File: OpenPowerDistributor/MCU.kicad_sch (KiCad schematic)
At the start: 1 part, among them U15 ESP32-S2-WROVER

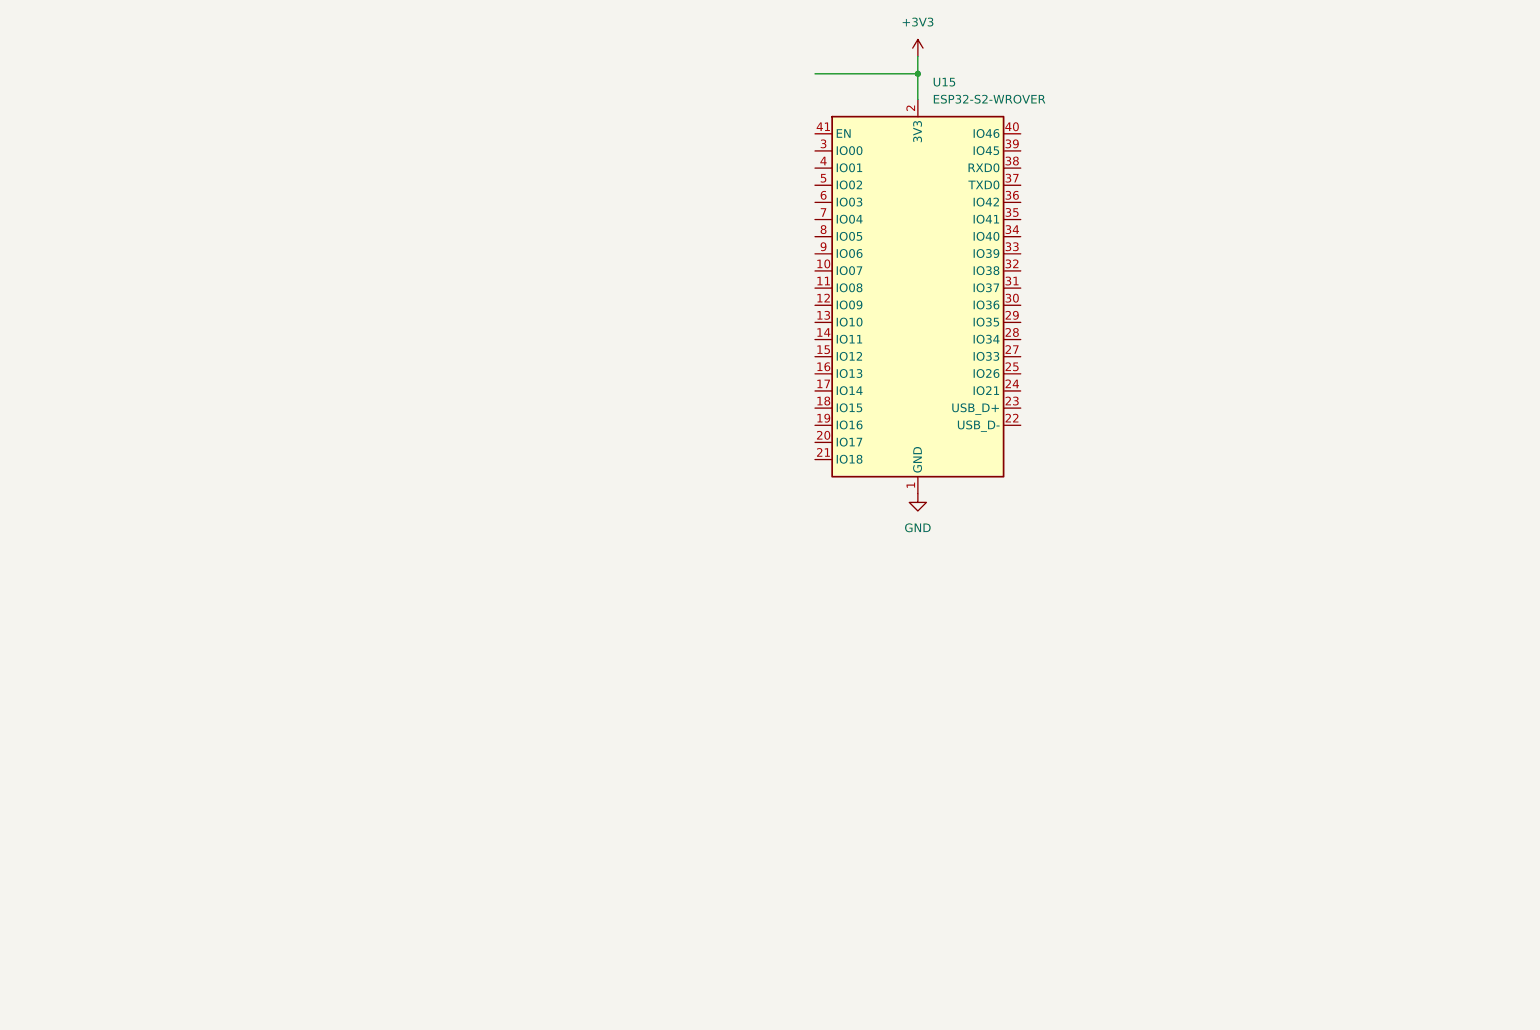
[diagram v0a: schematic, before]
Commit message: Analog multiplexer work
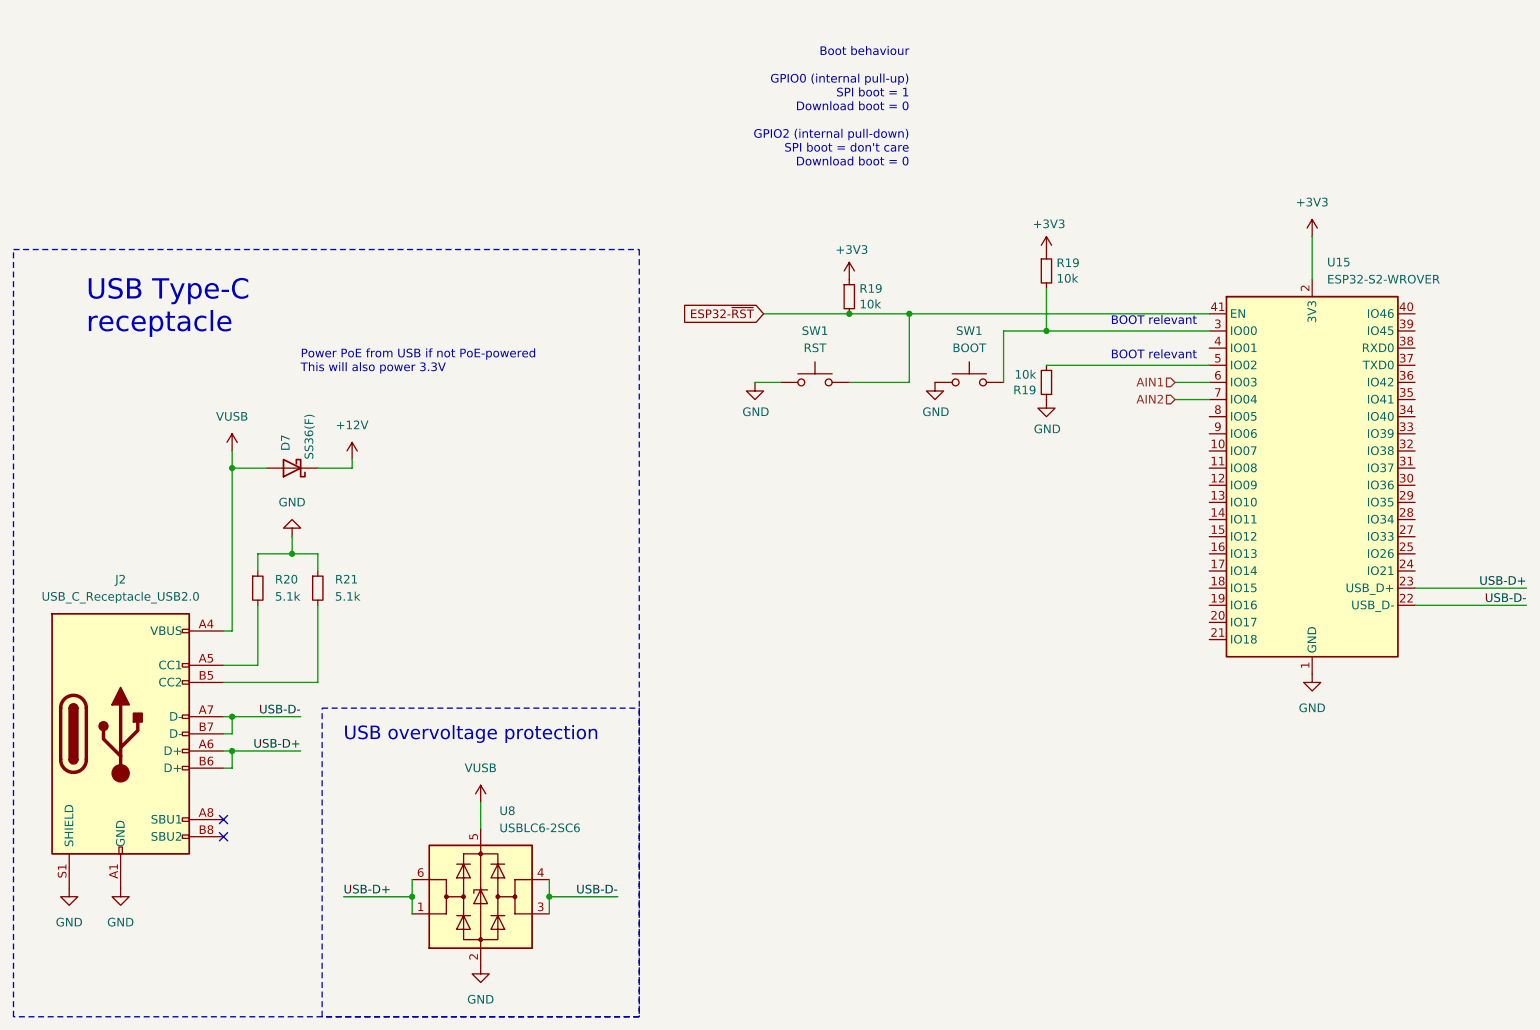
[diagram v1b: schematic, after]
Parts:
- added D7: SS36(F), Diode_SMD:D_SMA, symbol Device:D_Schottky
- added J2: USB_C_Receptacle_USB2.0, Connector_USB:USB_C_Receptacle_HCTL_HC-TYPE-C-16P-01A, symbol Connector:USB_C_Receptacle_USB2.0
- added R19 (x3): 10k, Resistor_SMD:R_0603_1608Metric, symbol Device:R_Small
- added R20, R21: 5.1k, Resistor_SMD:R_0603_1608Metric, symbol Device:R_Small
- added SW1: BOOT, Button_Switch_SMD:SW_SPST_TL3342, symbol Switch:SW_Push
- added SW1: RST, Button_Switch_SMD:SW_SPST_TL3342, symbol Switch:SW_Push
- added U8: USBLC6-2SC6, Package_TO_SOT_SMD:SOT-23-6, symbol Power_Protection:USBLC6-2SC6
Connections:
- net +3V3: now also R19.1, R19.1
- net GND: now also J2.A1 (GND), J2.A12 (GND), J2.B1 (GND), J2.B12 (GND), J2.S1 (SHIELD), R19.1, R20.1, R21.1, SW1.1, SW1.1, U8.2 (GND)
- net USB-D-: now reaches U15.22 (USB_D-)
- net USB-D-: now also J2.A7 (D-), J2.B7 (D-), U8.3 (I/O2), U8.4 (I/O2)
- net USB-D+: now reaches U15.23 (USB_D+)
- net USB-D+: now also J2.A6 (D+), J2.B6 (D+), U8.1 (I/O1), U8.6 (I/O1)
- net at U15.3 (IO00): now also R19.2, SW1.2
- net ESP32-~{RST}: now reaches U15.41 (EN)
- net ESP32-~{RST}: now also R19.2, SW1.2
- net at U15.5 (IO02): now also R19.2
- net AIN1: now reaches U15.6 (IO03)
- net AIN2: now reaches U15.7 (IO04)
- new net: J2.A5 (CC1), R20.2
- new net: J2.B5 (CC2), R21.2
- new net +12V: D7.1 (K)
- new net VUSB: D7.2 (A), J2.A4 (VBUS), J2.A9 (VBUS), J2.B4 (VBUS), J2.B9 (VBUS), U8.5 (VBUS)
- no-connect marks 0 -> 2
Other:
- note added: "BOOT relevant"
- note added: "Boot behaviour GPIO0 (internal pull-up) SPI boot = 1 Download boot = 0 GPIO2 (internal pull-down) SPI boot = don't care Download boot = 0"
- note added: "Power PoE from USB if not PoE-powered This will also power 3.3V"
- note added: "USB Type-C receptacle"
- note added: "USB overvoltage protection"
- moved on the sheet: U15
